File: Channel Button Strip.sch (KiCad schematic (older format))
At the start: 13 parts, among them J3 Conn_01x08_Male, J4 Conn_01x01_Male, J5 Conn_01x01_Male, J6 Conn_01x01_Male, J7 Conn_01x01_Male, SW33 SW_SPST_4_PIN, SW34 SW_SPST_4_PIN, SW35 SW_SPST_4_PIN, SW36 SW_SPST_4_PIN, SW37 SW_SPST_4_PIN, SW38 SW_SPST_4_PIN, SW39 SW_SPST_4_PIN, SW40 SW_SPST_4_PIN

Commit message: Further work on the separate boards
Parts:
- SW33, SW34, SW35, SW36, SW37, SW38, SW39, SW40: symbol sw_spst_0:SW_SPST_4_PIN -> cp_midi_control_surface_002-rescue:SW_SPST_4_PIN-sw_spst_0
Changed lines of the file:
@@
 $EndDescr
 $Comp
-L sw_spst_0:SW_SPST_4_PIN SW?
+L cp_midi_control_surface_002-rescue:SW_SPST_4_PIN-sw_spst_0 SW?
 U 1 1 5C4BA780
 P 2750 1900
 AR Path="/5C4B73B3/5C4BA780" Ref="SW?"  Part="1"
 AR Path="/5C4BA289/5C4BA780" Ref="SW33"  Part="1"
+AR Path="/5C4BA780" Ref="SW33"  Part="1"
 F 0 "SW33" H 2750 1700 50  0000 C CNN
 F 1 "SW_SPST_4_PIN" H 2750 2074 50  0001 C CNN
@@
 $EndComp
 $Comp
-L sw_spst_0:SW_SPST_4_PIN SW?
+L cp_midi_control_surface_002-rescue:SW_SPST_4_PIN-sw_spst_0 SW?
 U 1 1 5C4BA787
 P 2750 2400
 AR Path="/5C4B73B3/5C4BA787" Ref="SW?"  Part="1"
 AR Path="/5C4BA289/5C4BA787" Ref="SW34"  Part="1"
+AR Path="/5C4BA787" Ref="SW34"  Part="1"
 F 0 "SW34" H 2750 2200 50  0000 C CNN
 F 1 "SW_SPST_4_PIN" H 2750 2574 50  0001 C CNN
@@
 $EndComp
 $Comp
-L sw_spst_0:SW_SPST_4_PIN SW?
+L cp_midi_control_surface_002-rescue:SW_SPST_4_PIN-sw_spst_0 SW?
 U 1 1 5C4BA78E
 P 2750 2900
 AR Path="/5C4B73B3/5C4BA78E" Ref="SW?"  Part="1"
 AR Path="/5C4BA289/5C4BA78E" Ref="SW35"  Part="1"
+AR Path="/5C4BA78E" Ref="SW35"  Part="1"
 F 0 "SW35" H 2750 2700 50  0000 C CNN
 F 1 "SW_SPST_4_PIN" H 2750 3074 50  0001 C CNN
@@
 $EndComp
 $Comp
-L sw_spst_0:SW_SPST_4_PIN SW?
+L cp_midi_control_surface_002-rescue:SW_SPST_4_PIN-sw_spst_0 SW?
 U 1 1 5C4BA795
 P 2750 3400
 AR Path="/5C4B73B3/5C4BA795" Ref="SW?"  Part="1"
 AR Path="/5C4BA289/5C4BA795" Ref="SW36"  Part="1"
+AR Path="/5C4BA795" Ref="SW36"  Part="1"
 F 0 "SW36" H 2750 3200 50  0000 C CNN
 F 1 "SW_SPST_4_PIN" H 2750 3574 50  0001 C CNN
@@
 $EndComp
 $Comp
-L sw_spst_0:SW_SPST_4_PIN SW?
+L cp_midi_control_surface_002-rescue:SW_SPST_4_PIN-sw_spst_0 SW?
 U 1 1 5C4BA79C
 P 2750 3900
 AR Path="/5C4B73B3/5C4BA79C" Ref="SW?"  Part="1"
 AR Path="/5C4BA289/5C4BA79C" Ref="SW37"  Part="1"
+AR Path="/5C4BA79C" Ref="SW37"  Part="1"
 F 0 "SW37" H 2750 3700 50  0000 C CNN
 F 1 "SW_SPST_4_PIN" H 2750 4074 50  0001 C CNN
@@
 $EndComp
 $Comp
-L sw_spst_0:SW_SPST_4_PIN SW?
+L cp_midi_control_surface_002-rescue:SW_SPST_4_PIN-sw_spst_0 SW?
 U 1 1 5C4BA7A3
 P 2750 4400
 AR Path="/5C4B73B3/5C4BA7A3" Ref="SW?"  Part="1"
 AR Path="/5C4BA289/5C4BA7A3" Ref="SW38"  Part="1"
+AR Path="/5C4BA7A3" Ref="SW38"  Part="1"
 F 0 "SW38" H 2750 4200 50  0000 C CNN
 F 1 "SW_SPST_4_PIN" H 2750 4574 50  0001 C CNN
@@
 $EndComp
 $Comp
-L sw_spst_0:SW_SPST_4_PIN SW?
+L cp_midi_control_surface_002-rescue:SW_SPST_4_PIN-sw_spst_0 SW?
 U 1 1 5C4BA7AA
 P 2750 4900
 AR Path="/5C4B73B3/5C4BA7AA" Ref="SW?"  Part="1"
 AR Path="/5C4BA289/5C4BA7AA" Ref="SW39"  Part="1"
+AR Path="/5C4BA7AA" Ref="SW39"  Part="1"
 F 0 "SW39" H 2750 4700 50  0000 C CNN
 F 1 "SW_SPST_4_PIN" H 2750 5074 50  0001 C CNN
@@
 $EndComp
 $Comp
-L sw_spst_0:SW_SPST_4_PIN SW?
+L cp_midi_control_surface_002-rescue:SW_SPST_4_PIN-sw_spst_0 SW?
 U 1 1 5C4BA7B1
 P 2750 5400
 AR Path="/5C4B73B3/5C4BA7B1" Ref="SW?"  Part="1"
 AR Path="/5C4BA289/5C4BA7B1" Ref="SW40"  Part="1"
+AR Path="/5C4BA7B1" Ref="SW40"  Part="1"
 F 0 "SW40" H 2750 5200 50  0000 C CNN
 F 1 "SW_SPST_4_PIN" H 2750 5574 50  0001 C CNN

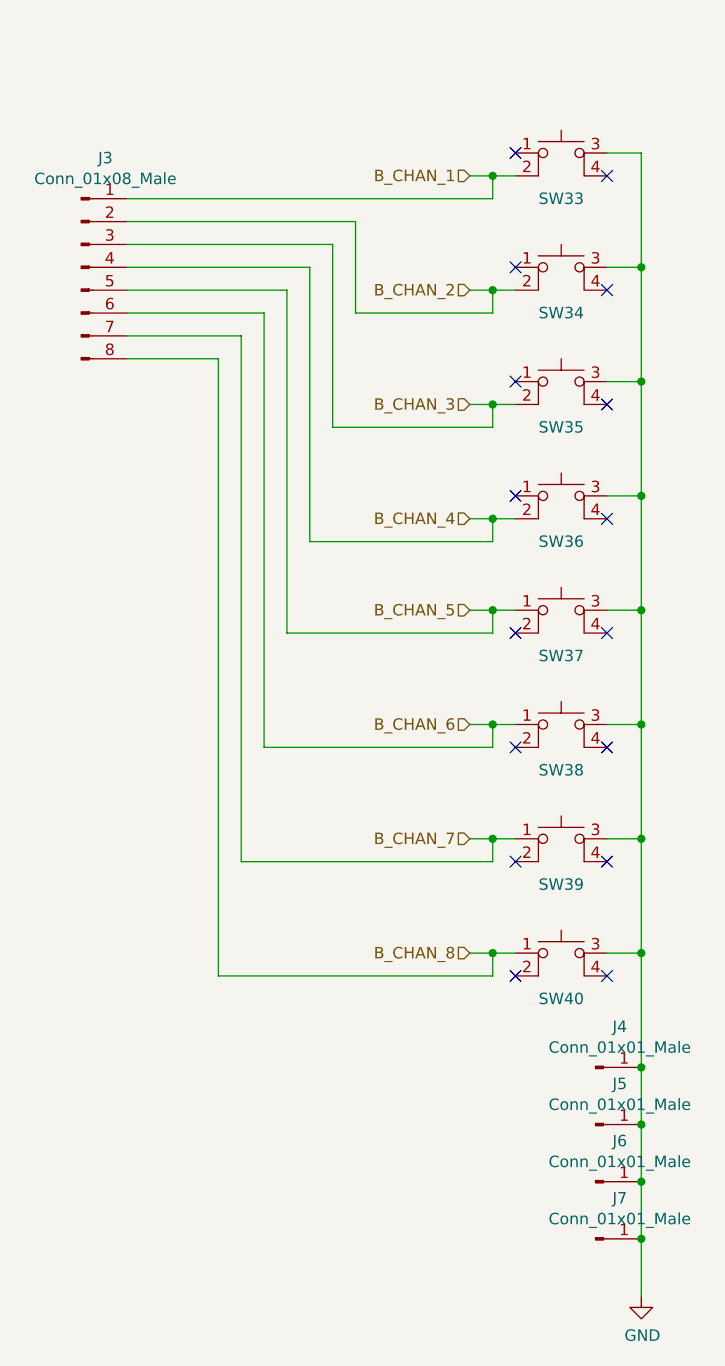
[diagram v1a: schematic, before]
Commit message: Sub boards completed
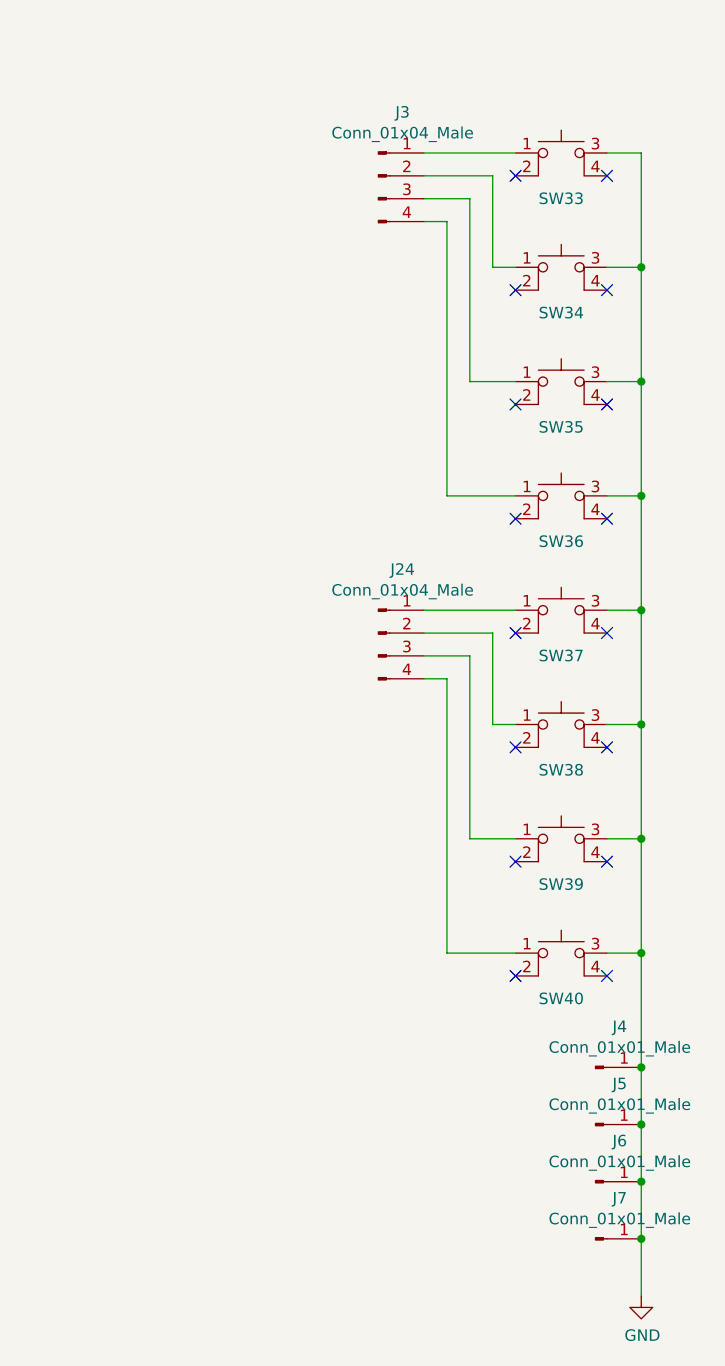
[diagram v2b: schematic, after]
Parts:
- removed J3: Conn_01x08_Male, Connector_PinHeader_2.54mm:PinHeader_1x08_P2.54mm_Vertical, symbol Connector:Conn_01x08_Male
- added J24, J3: Conn_01x04_Male, Connector_PinHeader_2.54mm:PinHeader_1x04_P2.54mm_Vertical, symbol Connector:Conn_01x04_Male
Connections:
- net at SW33.1 (A): now also J3.1 (Pin_1)
- net at SW34.1 (A): now also J3.2 (Pin_2)
- net at SW35.1 (A): now also J3.3 (Pin_3)
- net at SW36.1 (A): now also J3.4 (Pin_4)
- net B_CHAN_1: no longer names the net of SW33.2
- net B_CHAN_2: no longer names the net of SW34.2
- net B_CHAN_3: no longer names the net of SW35.2
- net B_CHAN_4: no longer names the net of SW36.2
- net B_CHAN_5: no longer names the net of SW37.1 (A)
- net B_CHAN_5: now also J24.1 (Pin_1)
- net B_CHAN_6: no longer names the net of SW38.1 (A)
- net B_CHAN_6: now also J24.2 (Pin_2)
- net B_CHAN_7: no longer names the net of SW39.1 (A)
- net B_CHAN_7: now also J24.3 (Pin_3)
- net B_CHAN_8: no longer names the net of SW40.1 (A)
- net B_CHAN_8: now also J24.4 (Pin_4)
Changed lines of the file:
@@
 Wire Wire Line
 	3100 2400 3100 2900
-Text HLabel 2350 2000 0    50   Input ~ 0
-B_CHAN_1
-Text HLabel 2350 2500 0    50   Input ~ 0
-B_CHAN_2
-Text HLabel 2350 3000 0    50   Input ~ 0
-B_CHAN_3
-Text HLabel 2350 3500 0    50   Input ~ 0
-B_CHAN_4
-Text HLabel 2350 3900 0    50   Input ~ 0
-B_CHAN_5
-Text HLabel 2350 4400 0    50   Input ~ 0
-B_CHAN_6
-Text HLabel 2350 4900 0    50   Input ~ 0
-B_CHAN_7
-Text HLabel 2350 5400 0    50   Input ~ 0
-B_CHAN_8
-Wire Wire Line
-	2350 2000 2450 2000
-Wire Wire Line
-	2350 2500 2450 2500
-Wire Wire Line
-	2350 3000 2450 3000
-Wire Wire Line
-	2350 3500 2450 3500
-Wire Wire Line
-	2350 3900 2450 3900
-Wire Wire Line
-	2350 4400 2450 4400
-Wire Wire Line
-	2350 4900 2450 4900
-Wire Wire Line
-	2350 5400 2450 5400
 NoConn ~ 2950 2000
 NoConn ~ 2950 2500
@@
 NoConn ~ 2550 5500
 NoConn ~ 2950 5500
-NoConn ~ 2550 1900
-NoConn ~ 2550 2400
-NoConn ~ 2550 2900
-NoConn ~ 2550 3400
-$Comp
-L Connector:Conn_01x08_Male J3
-U 1 1 5CBFD5BE
-P 650 2400
-F 0 "J3" H 756 2878 50  0000 C CNN
-F 1 "Conn_01x08_Male" H 756 2787 50  0000 C CNN
-F 2 "Connector_PinHeader_2.54mm:PinHeader_1x08_P2.54mm_Vertical" H 650 2400 50  0001 C CNN
-F 3 "~" H 650 2400 50  0001 C CNN
-	1    650  2400
-	1    0    0    -1
-$EndComp
-Wire Wire Line
-	2450 2000 2450 2100
-Wire Wire Line
-	2450 2100 850  2100
-Connection ~ 2450 2000
-Wire Wire Line
-	2450 2000 2550 2000
-Wire Wire Line
-	2450 2500 2450 2600
-Wire Wire Line
-	2450 2600 1850 2600
-Wire Wire Line
-	1850 2600 1850 2200
-Wire Wire Line
-	1850 2200 850  2200
-Connection ~ 2450 2500
-Wire Wire Line
-	2450 2500 2550 2500
-Wire Wire Line
-	850  2300 1750 2300
-Wire Wire Line
-	1750 2300 1750 3100
-Wire Wire Line
-	1750 3100 2450 3100
-Wire Wire Line
-	2450 3100 2450 3000
-Connection ~ 2450 3000
-Wire Wire Line
-	2450 3000 2550 3000
-Wire Wire Line
-	850  2400 1650 2400
-Wire Wire Line
-	1650 2400 1650 3600
-Wire Wire Line
-	1650 3600 2450 3600
-Wire Wire Line
-	2450 3600 2450 3500
-Connection ~ 2450 3500
-Wire Wire Line
-	2450 3500 2550 3500
-Wire Wire Line
-	850  2500 1550 2500
-Wire Wire Line
-	1550 2500 1550 4000
-Wire Wire Line
-	1550 4000 2450 4000
-Wire Wire Line
-	2450 4000 2450 3900
-Connection ~ 2450 3900
-Wire Wire Line
-	2450 3900 2550 3900
-Wire Wire Line
-	850  2600 1450 2600
-Wire Wire Line
-	1450 2600 1450 4500
-Wire Wire Line
-	1450 4500 2450 4500
-Wire Wire Line
-	2450 4500 2450 4400
-Connection ~ 2450 4400
-Wire Wire Line
-	2450 4400 2550 4400
-Wire Wire Line
-	850  2700 1350 2700
-Wire Wire Line
-	1350 2700 1350 5000
-Wire Wire Line
-	1350 5000 2450 5000
-Wire Wire Line
-	2450 5000 2450 4900
-Connection ~ 2450 4900
-Wire Wire Line
-	2450 4900 2550 4900
-Wire Wire Line
-	850  2800 1250 2800
-Wire Wire Line
-	1250 2800 1250 5500
-Wire Wire Line
-	1250 5500 2450 5500
-Wire Wire Line
-	2450 5500 2450 5400
-Connection ~ 2450 5400
-Wire Wire Line
-	2450 5400 2550 5400
 $Comp
 L Connector:Conn_01x01_Male J7
@@
 	3100 6650 3100 6900
 Connection ~ 3100 6650
+$Comp
+L Connector:Conn_01x04_Male J3
+U 1 1 5C755D1C
+P 1950 2000
+F 0 "J3" H 2056 2278 50  0000 C CNN
+F 1 "Conn_01x04_Male" H 2056 2187 50  0000 C CNN
+F 2 "Connector_PinHeader_2.54mm:PinHeader_1x04_P2.54mm_Vertical" H 1950 2000 50  0001 C CNN
+F 3 "~" H 1950 2000 50  0001 C CNN
+	1    1950 2000
+	1    0    0    -1
+$EndComp
+$Comp
+L Connector:Conn_01x04_Male J24
+U 1 1 5C756AEE
+P 1950 4000
+F 0 "J24" H 2056 4278 50  0000 C CNN
+F 1 "Conn_01x04_Male" H 2056 4187 50  0000 C CNN
+F 2 "Connector_PinHeader_2.54mm:PinHeader_1x04_P2.54mm_Vertical" H 1950 4000 50  0001 C CNN
+F 3 "~" H 1950 4000 50  0001 C CNN
+	1    1950 4000
+	1    0    0    -1
+$EndComp
+Wire Wire Line
+	2550 4400 2450 4400
+Wire Wire Line
+	2450 4400 2450 4000
+Wire Wire Line
+	2550 4900 2350 4900
+Wire Wire Line
+	2350 4900 2350 4100
+Wire Wire Line
+	2550 5400 2250 5400
+Wire Wire Line
+	2250 5400 2250 4200
+Wire Wire Line
+	2250 4200 2150 4200
+Wire Wire Line
+	2350 4100 2150 4100
+Wire Wire Line
+	2450 4000 2150 4000
+Wire Wire Line
+	2550 3900 2150 3900
+Wire Wire Line
+	2550 1900 2150 1900
+Wire Wire Line
+	2550 2400 2450 2400
+Wire Wire Line
+	2450 2400 2450 2000
+Wire Wire Line
+	2450 2000 2150 2000
+Wire Wire Line
+	2550 2900 2350 2900
+Wire Wire Line
+	2350 2900 2350 2100
+Wire Wire Line
+	2350 2100 2150 2100
+Wire Wire Line
+	2550 3400 2250 3400
+Wire Wire Line
+	2250 3400 2250 2200
+Wire Wire Line
+	2250 2200 2150 2200
+NoConn ~ 2550 2000
+NoConn ~ 2550 2500
+NoConn ~ 2550 3000
+NoConn ~ 2550 3500
 $EndSCHEMATC
